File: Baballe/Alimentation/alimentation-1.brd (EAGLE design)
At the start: 30 x 30 mm, 17 parts, among them Q1 2.5A/30V, U1 MCP73831, U2 3.3V

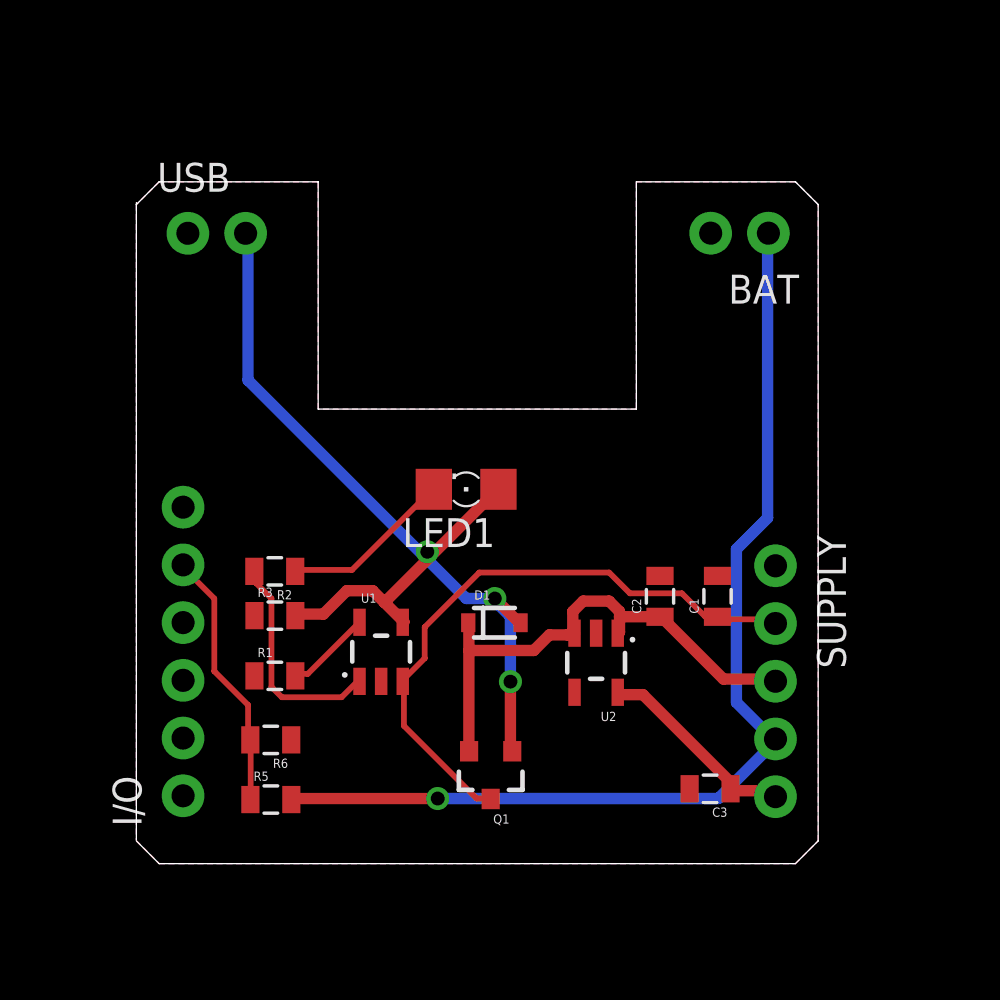
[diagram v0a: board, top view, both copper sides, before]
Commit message: V2 de la Baballe
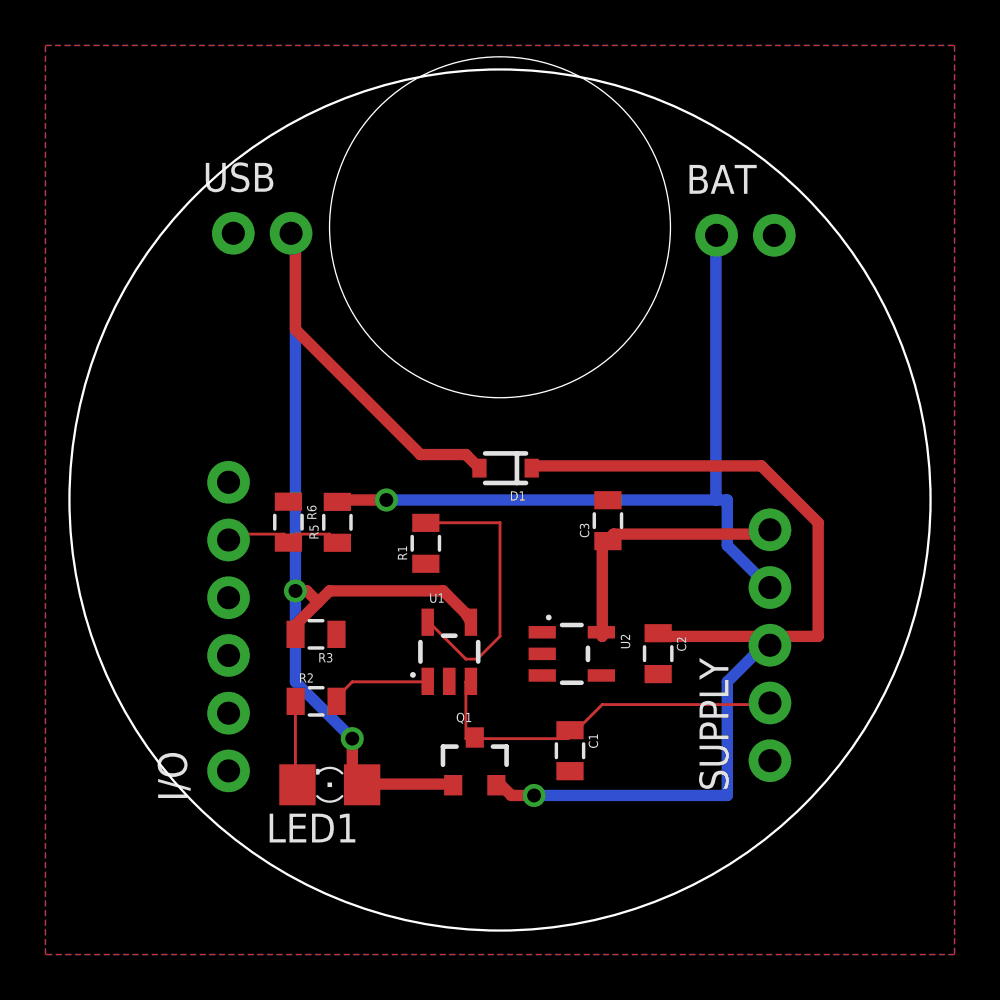
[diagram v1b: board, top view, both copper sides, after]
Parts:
- moved LED1 14.3 mm to (8.51, 55.5)
- moved C3 12.6 mm to (20.7, 67.1), turned to 90 degrees
- moved R5 12.5 mm to (8.85, 67.0), turned to 90 degrees
- moved R6 9.61 mm to (6.69, 67.0), turned to 270 degrees
- moved C1 9.39 mm to (19.1, 57.0), turned to 270 degrees
- moved R1 8.84 mm to (12.7, 66.1), turned to 90 degrees
- moved SUPPLY 8.58 mm to (27.9, 56.5), turned to 90 degrees
- moved D1 6.82 mm to (16.2, 69.4), turned to 180 degrees
- moved R2 6.00 mm to (7.91, 59.1), turned to 0 degrees
- moved U1 3.00 mm to (13.8, 61.3)
- moved C2 2.52 mm to (23.0, 61.2), turned to 270 degrees
- moved BAT 2.28 mm to (25.5, 79.6), turned to 0 degrees
- moved I/O 2.28 mm to (4.06, 56.1)
- moved USB 2.00 mm to (4.27, 79.7)
- moved R3 1.99 mm to (7.90, 62.1), turned to 180 degrees
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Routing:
- net VIN: track 23.1 -> 44.3 mm, vias 0 -> 1
- net V_BATT: track 46.1 -> 33.5 mm
- net VUSB: track 43.4 -> 55.4 mm, vias 3 -> 2
- net VCC_2: track 27.4 -> 16.9 mm
- net N$2: track 3.80 -> 12.5 mm
- net V_BAT_MESURE: track 11.6 -> 5.44 mm
- net N$4: track 9.75 -> 4.80 mm
- net N$1: track 7.58 -> 3.73 mm
- net VCC: track 9.08 -> 11.8 mm
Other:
- board size 30 x 30 mm -> 37.9 x 37.9 mm
